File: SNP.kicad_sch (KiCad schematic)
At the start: 10 parts, among them J1 SNP, SW1 Reset button, U75 IN74ALS32N (КР1533ЛЛ1)

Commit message: March 26th update
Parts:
- J1: footprint zxspectrum:SNP96 -> w_conn_av:snp59_96_female_angle_2
- U75: footprint Package_DIP:DIP-14_W7.62mm_Socket_LongPads -> Package_DIP:DIP-14_W7.62mm_Socket
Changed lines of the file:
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@@
     (property "Reference" "U75" (id 0) (at 150.495 134.62 0))
     (property "Value" "IN74ALS32N (КР1533ЛЛ1)" (id 1) (at 149.86 127.635 0))
-    (property "Footprint" "Package_DIP:DIP-14_W7.62mm_Socket_LongPads" (id 2) (at 149.86 134.62 0)
+    (property "Footprint" "Package_DIP:DIP-14_W7.62mm_Socket" (id 2) (at 149.86 134.62 0)
       (effects (font (size 1.27 1.27)) hide)
     )
@@
     (property "Reference" "J1" (id 0) (at 53.34 26.035 0))
     (property "Value" "SNP" (id 1) (at 53.34 28.575 0))
-    (property "Footprint" "zxspectrum:SNP96" (id 2) (at 53.34 27.94 0)
+    (property "Footprint" "w_conn_av:snp59_96_female_angle_2" (id 2) (at 53.34 27.94 0)
       (effects (font (size 1.27 1.27)) hide)
     )
@@
     (property "Reference" "U75" (id 0) (at 130.175 132.08 0))
     (property "Value" "IN74ALS32N (КР1533ЛЛ1)" (id 1) (at 130.175 125.73 0))
-    (property "Footprint" "Package_DIP:DIP-14_W7.62mm_Socket_LongPads" (id 2) (at 130.175 132.08 0)
+    (property "Footprint" "Package_DIP:DIP-14_W7.62mm_Socket" (id 2) (at 130.175 132.08 0)
       (effects (font (size 1.27 1.27)) hide)
     )

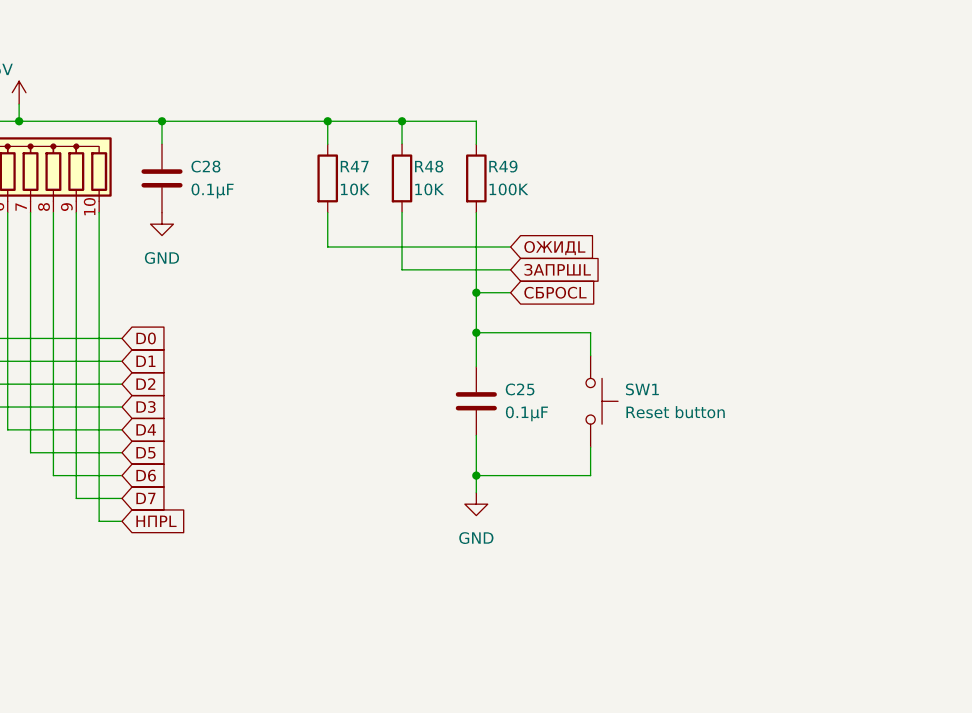
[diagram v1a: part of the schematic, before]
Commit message: 28th march ver2
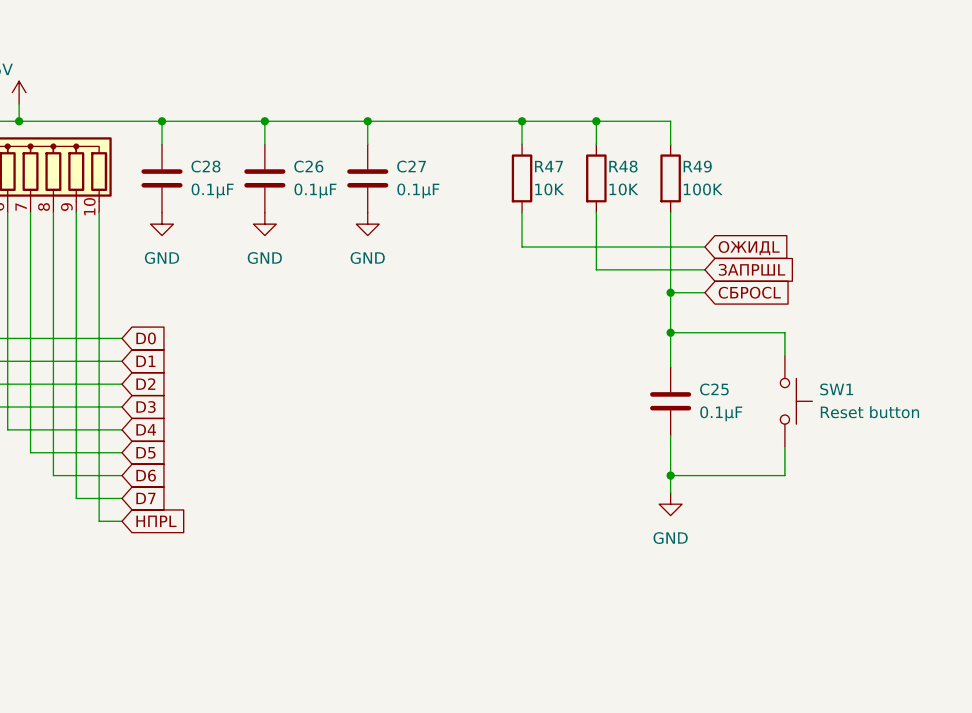
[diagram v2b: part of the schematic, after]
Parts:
- added C26, C27: 0.1μF, Capacitor_THT:C_Disc_D7.0mm_W2.5mm_P5.00mm, symbol Device:C
- J1: footprint w_conn_av:snp59_96_female_angle_2 -> delta:snp59_96_female_angle_3
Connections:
- net +5V: now also C26.1, C27.1
- net GND: now also C26.2, C27.2
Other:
- moved on the sheet: C25, R47, R48, R49, SW1
